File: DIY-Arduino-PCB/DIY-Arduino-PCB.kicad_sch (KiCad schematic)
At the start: 29 parts, among them J1 USB_C_Receptacle_USB2.0_16P, SW1 SW_Push, U5 ATmega328P-M, U6 CH340G, Y2 Crystal, Y3 Crystal

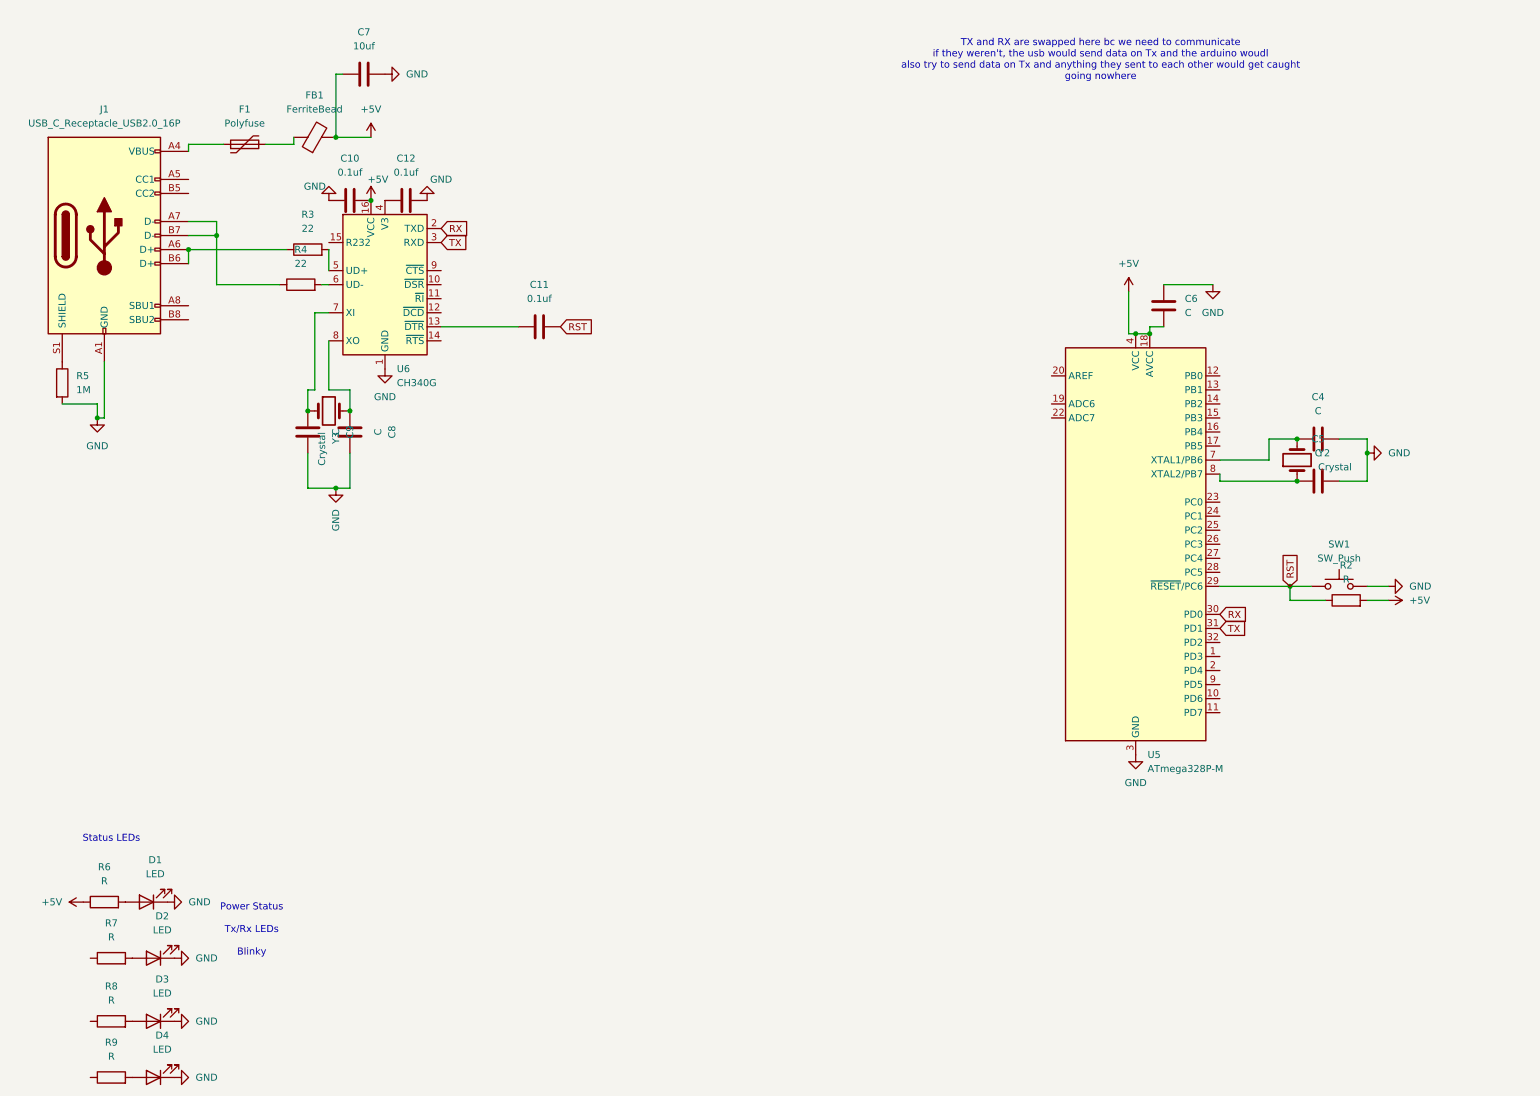
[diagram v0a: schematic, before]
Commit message: made some progress. Some odds and ends.
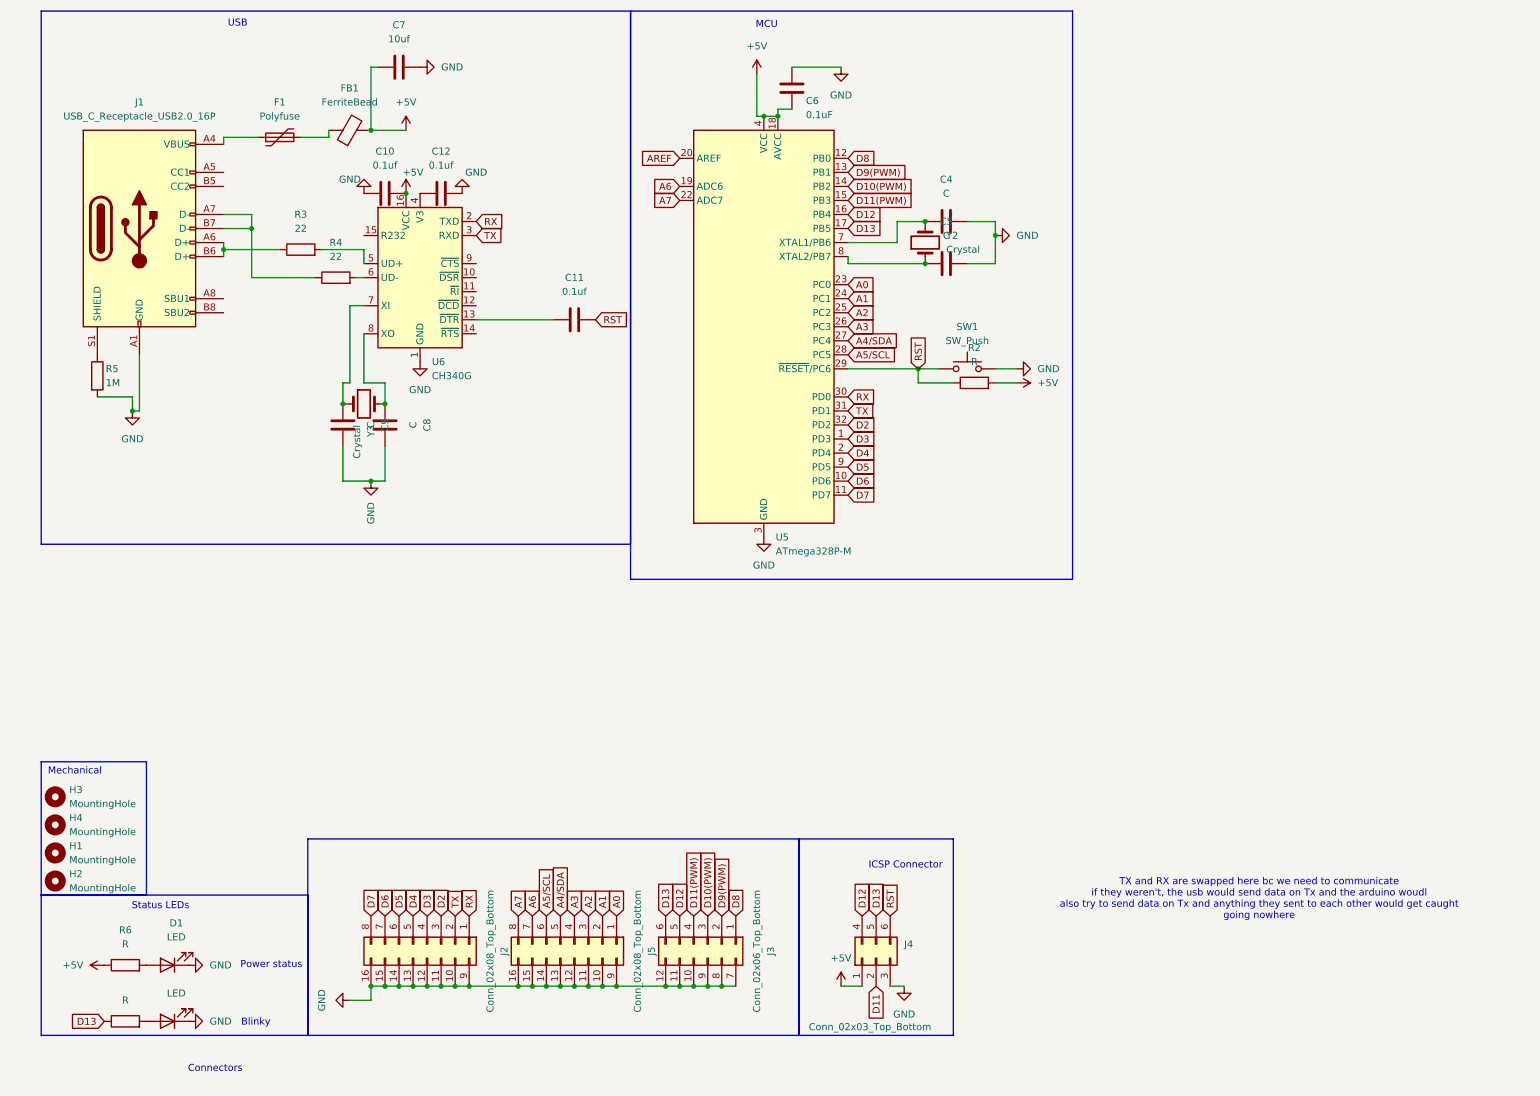
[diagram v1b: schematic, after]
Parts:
- removed D2, D3: LED, symbol Device:LED
- removed R7, R8: R, symbol Device:R
- added H1, H2, H3, H4: MountingHole, symbol Mechanical:MountingHole
- added J2, J5: Conn_02x08_Top_Bottom, Connector_JAE:JAE_LY20-16P-DLT1_2x08_P2.00mm_Horizontal, symbol Connector_Generic:Conn_02x08_Top_Bottom
- added J3: Conn_02x06_Top_Bottom, symbol Connector_Generic:Conn_02x06_Top_Bottom
- added J4: Conn_02x03_Top_Bottom, symbol Connector_Generic:Conn_02x03_Top_Bottom
- C6: value C -> 0.1uF
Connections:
- net +5V: now also J4.1 (Pin_1)
- net GND: now also J2.10 (Pin_10), J2.11 (Pin_11), J2.12 (Pin_12), J2.13 (Pin_13), J2.14 (Pin_14), J2.15 (Pin_15), J2.16 (Pin_16), J2.9 (Pin_9), J3.10 (Pin_10), J3.11 (Pin_11), J3.12 (Pin_12), J3.7 (Pin_7), J3.8 (Pin_8), J3.9 (Pin_9), J4.3 (Pin_3), J5.10 (Pin_10), J5.11 (Pin_11), J5.12 (Pin_12), J5.13 (Pin_13), J5.14 (Pin_14), J5.15 (Pin_15), J5.16 (Pin_16), J5.9 (Pin_9)
- net RST: now also J4.6 (Pin_6)
- net RX: now also J2.1 (Pin_1)
- net TX: now also J2.2 (Pin_2)
- net D13: now reaches R9.1
- net D13: now also U5.17 (PB5), J3.6 (Pin_6), J4.5 (Pin_5)
- net D3: now reaches U5.1 (PD3)
- net D3: now also J2.4 (Pin_4)
- net D6: now reaches U5.10 (PD6)
- net D6: now also J2.7 (Pin_7)
- net D7: now reaches U5.11 (PD7)
- net D7: now also J2.8 (Pin_8)
- net D8: now reaches U5.12 (PB0)
- net D8: now also J3.1 (Pin_1)
- net D9(PWM): now reaches U5.13 (PB1)
- net D9(PWM): now also J3.2 (Pin_2)
- net D10(PWM): now reaches U5.14 (PB2)
- net D10(PWM): now also J3.3 (Pin_3)
- net D11(PWM): now reaches U5.15 (PB3)
- net D11(PWM): now also J3.4 (Pin_4)
- net D12: now reaches U5.16 (PB4)
- net D12: now also J3.5 (Pin_5), J4.4 (Pin_4)
- net A6: now reaches U5.19 (ADC6)
- net A6: now also J5.7 (Pin_7)
- net D4: now reaches U5.2 (PD4)
- net D4: now also J2.5 (Pin_5)
- net AREF: now reaches U5.20 (AREF)
- net A7: now reaches U5.22 (ADC7)
- net A7: now also J5.8 (Pin_8)
- net A0: now reaches U5.23 (PC0)
- net A0: now also J5.1 (Pin_1)
- net A1: now reaches U5.24 (PC1)
- net A1: now also J5.2 (Pin_2)
- net A2: now reaches U5.25 (PC2)
- net A2: now also J5.3 (Pin_3)
- net A3: now reaches U5.26 (PC3)
- net A3: now also J5.4 (Pin_4)
- net A4/SDA: now reaches U5.27 (PC4)
- net A4/SDA: now also J5.5 (Pin_5)
- net A5/SCL: now reaches U5.28 (PC5)
- net A5/SCL: now also J5.6 (Pin_6)
- net D2: now reaches U5.32 (PD2)
- net D2: now also J2.3 (Pin_3)
- net D5: now reaches U5.9 (PD5)
- net D5: now also J2.6 (Pin_6)
- new net D11: J4.2 (Pin_2)
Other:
- note added: "Blinky"
- note added: "Connectors"
- note added: "ICSP Connector"
- note added: "MCU"
- note added: "Mechanical"
- note added: "Power status"
- note added: "USB"
- note removed: "Power Status Tx/Rx LEDs Blinky"
- moved on the sheet: C10, C11, C12, C4, C5, C6, C7, C8, C9, D1, F1, FB1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
